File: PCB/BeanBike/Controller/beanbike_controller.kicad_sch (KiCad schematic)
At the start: 14 parts, among them SW1 SW_SPDT, U4 STM32G473RETx

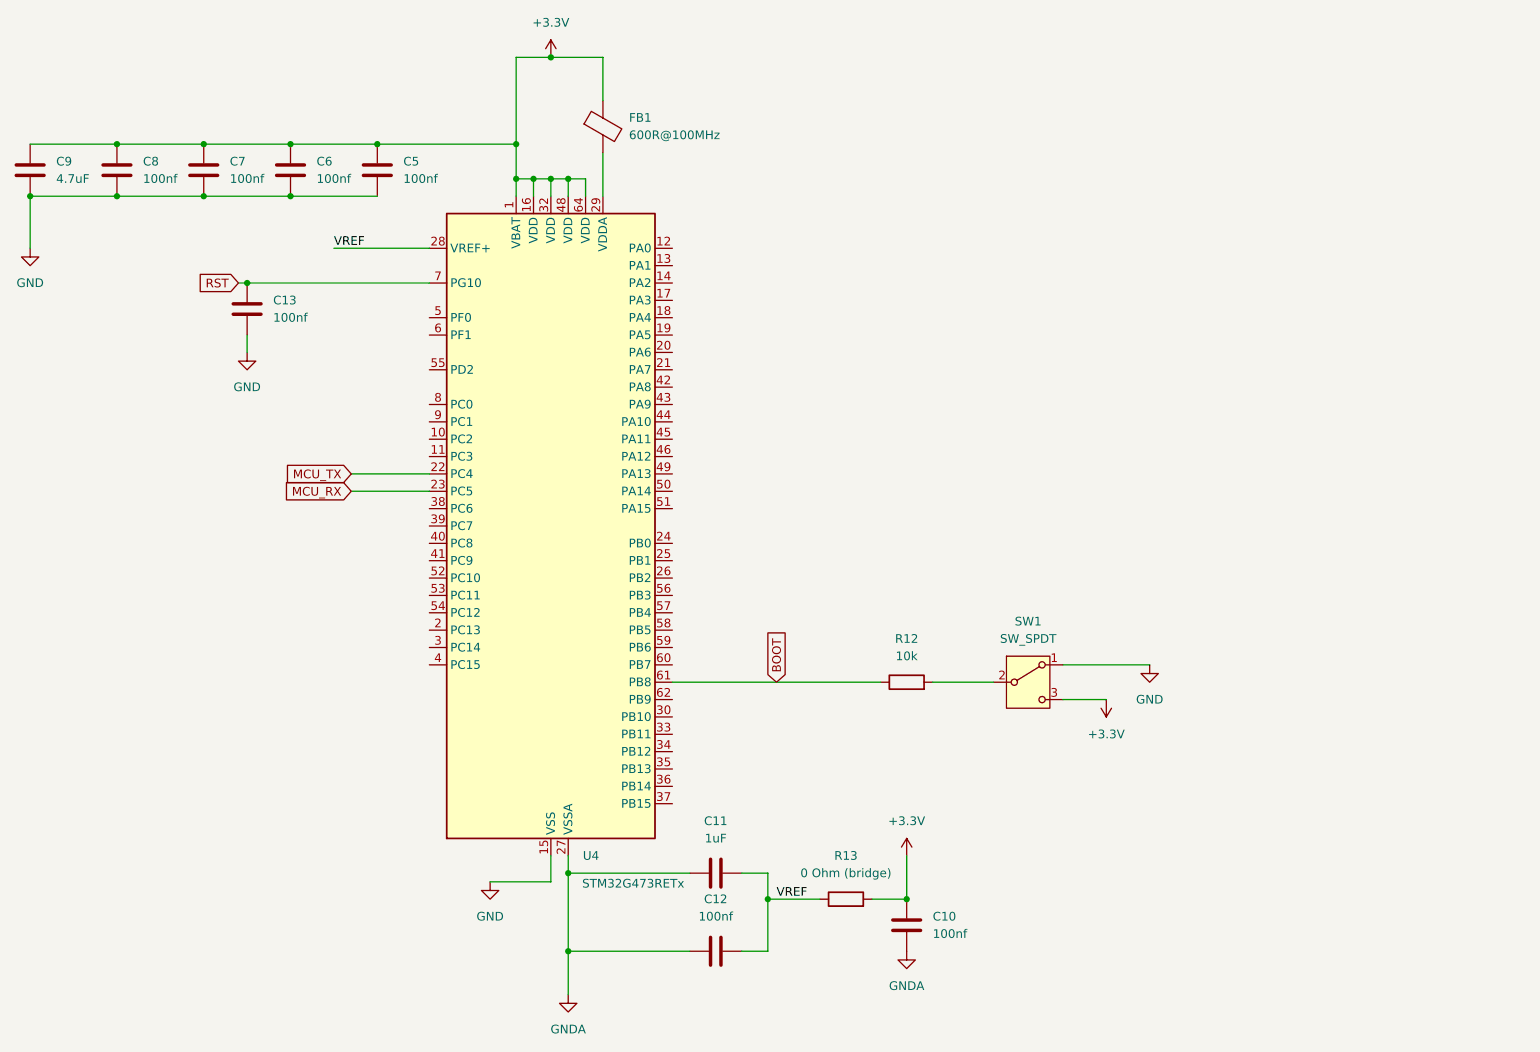
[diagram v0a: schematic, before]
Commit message: CAN
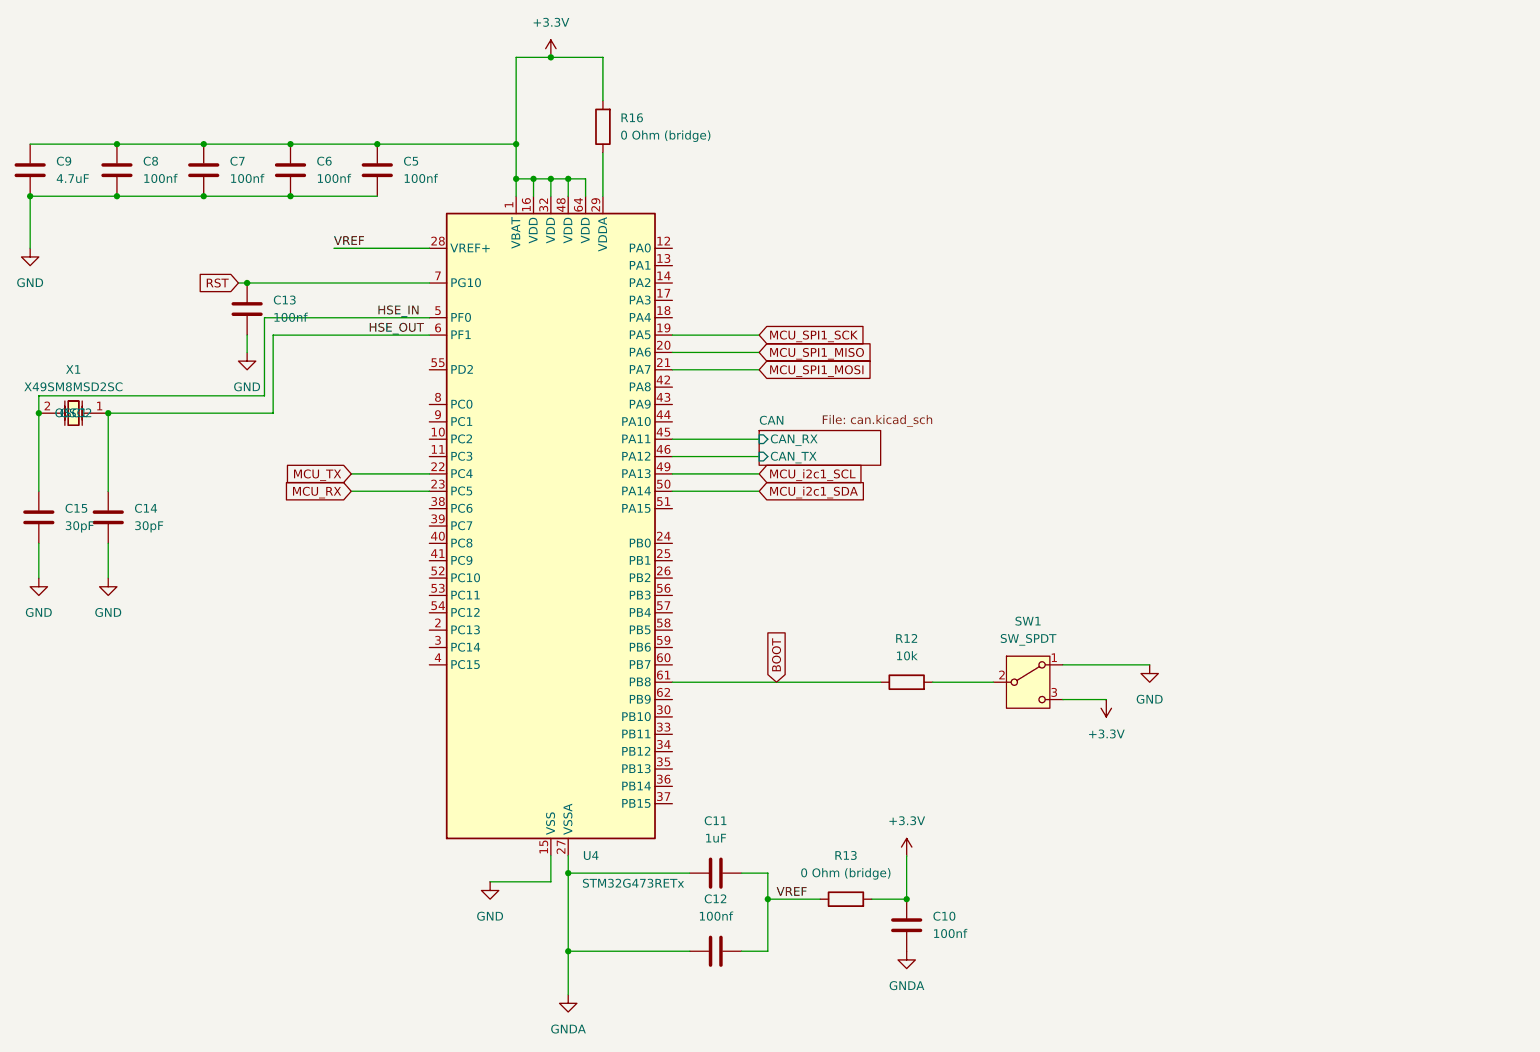
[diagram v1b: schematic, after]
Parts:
- removed FB1: 600R@100MHz, symbol Device:FerriteBead
- added C14, C15: 30pF, symbol Device:C
- added R16: 0 Ohm (bridge), symbol Device:R
- added X1: X49SM8MSD2SC, easyeda2kicad:CRYSTAL-SMD_L11.5-W4.8-LS12.7, symbol easyeda2kicad:X49SM8MSD2SC
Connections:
- net +3.3V: now also R16.2
- net GND: now also C14.2, C15.2
- net MCU_SPI1_SCK: now reaches U4.19 (PA5)
- net MCU_SPI1_MISO: now reaches U4.20 (PA6)
- net MCU_SPI1_MOSI: now reaches U4.21 (PA7)
- net at U4.29 (VDDA): now also R16.1
- net CAN/CAN_RX: now reaches U4.45 (PA11)
- net CAN/CAN_TX: now reaches U4.46 (PA12)
- net MCU_i2c1_SCL: now reaches U4.49 (PA13)
- net HSE_IN: now reaches U4.5 (PF0)
- net HSE_IN: now also C15.1, X1.2 (OSC2)
- net MCU_i2c1_SDA: now reaches U4.50 (PA14)
- net HSE_OUT: now reaches U4.6 (PF1)
- net HSE_OUT: now also C14.1, X1.1 (OSC1)
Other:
- added sheet CAN (can.kicad_sch)

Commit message: Schematic v3 Done
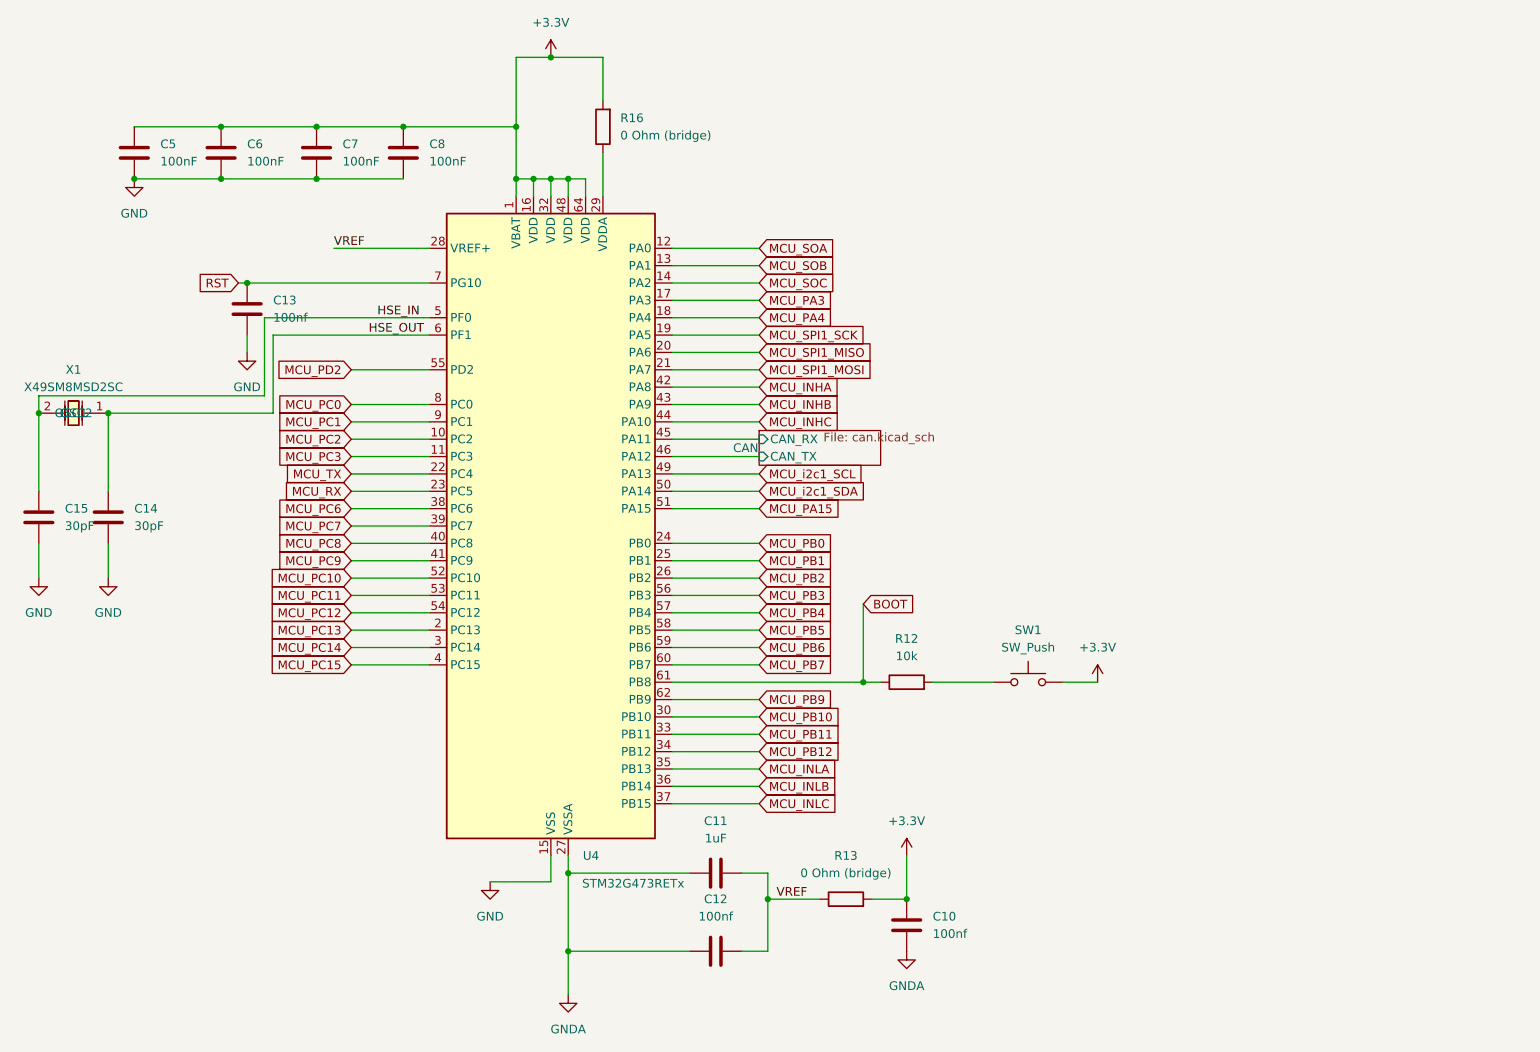
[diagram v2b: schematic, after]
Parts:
- removed C9: 4.7uF, symbol Device:C
- removed SW1: SW_SPDT, symbol Switch:SW_SPDT
- added SW1: SW_Push, symbol Switch:SW_Push
- C5, C6, C7, C8: value 100nf -> 100nF
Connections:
- net +3.3V: now also C5.2, C6.2, C7.2, C8.2, SW1.2; no longer C5.1, C6.1, C7.1, C8.1
- net GND: now also C5.1, C6.1, C7.1, C8.1; no longer C5.2, C6.2, C7.2, C8.2
- net at R12.2: now also SW1.1
- net MCU_PC2: now reaches U4.10 (PC2)
- net MCU_PC3: now reaches U4.11 (PC3)
- net MCU_SOA: now reaches U4.12 (PA0)
- net MCU_SOB: now reaches U4.13 (PA1)
- net MCU_SOC: now reaches U4.14 (PA2)
- net MCU_PA3: now reaches U4.17 (PA3)
- net MCU_PA4: now reaches U4.18 (PA4)
- net MCU_PC13: now reaches U4.2 (PC13)
- net MCU_PB0: now reaches U4.24 (PB0)
- net MCU_PB1: now reaches U4.25 (PB1)
- net MCU_PB2: now reaches U4.26 (PB2)
- net MCU_PC14: now reaches U4.3 (PC14)
- net MCU_PB10: now reaches U4.30 (PB10)
- net MCU_PB11: now reaches U4.33 (PB11)
- net MCU_PB12: now reaches U4.34 (PB12)
- net MCU_INLA: now reaches U4.35 (PB13)
- net MCU_INLB: now reaches U4.36 (PB14)
- net MCU_INLC: now reaches U4.37 (PB15)
- net MCU_PC6: now reaches U4.38 (PC6)
- net MCU_PC7: now reaches U4.39 (PC7)
- net MCU_PC15: now reaches U4.4 (PC15)
- net MCU_PC8: now reaches U4.40 (PC8)
- net MCU_PC9: now reaches U4.41 (PC9)
- net MCU_INHA: now reaches U4.42 (PA8)
- net MCU_INHB: now reaches U4.43 (PA9)
- net MCU_INHC: now reaches U4.44 (PA10)
- net MCU_PA15: now reaches U4.51 (PA15)
- net MCU_PC10: now reaches U4.52 (PC10)
- net MCU_PC11: now reaches U4.53 (PC11)
- net MCU_PC12: now reaches U4.54 (PC12)
- net MCU_PD2: now reaches U4.55 (PD2)
- net MCU_PB3: now reaches U4.56 (PB3)
- net MCU_PB4: now reaches U4.57 (PB4)
- net MCU_PB5: now reaches U4.58 (PB5)
- net MCU_PB6: now reaches U4.59 (PB6)
- net MCU_PB7: now reaches U4.60 (PB7)
- net MCU_PB9: now reaches U4.62 (PB9)
- net MCU_PC0: now reaches U4.8 (PC0)
- net MCU_PC1: now reaches U4.9 (PC1)

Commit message: Footprints
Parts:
- C10, C12, C13, C5, C6, C7, C8: footprint (none) -> Capacitor_SMD:C_0402_1005Metric; LCSC (none) -> C1525
- C11: footprint (none) -> Capacitor_SMD:C_0402_1005Metric; LCSC (none) -> C52923
- C14, C15: footprint (none) -> Capacitor_SMD:C_0402_1005Metric; LCSC (none) -> C1570
- R12: footprint (none) -> Resistor_SMD:R_0805_2012Metric; LCSC (none) -> C17414
- R13, R16: footprint (none) -> Resistor_SMD:R_0805_2012Metric; LCSC (none) -> C17477
- SW1: footprint (none) -> easyeda2kicad:SW-SMD_L3.9-W3.0-P4.45; LCSC (none) -> C720477
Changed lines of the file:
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@@
 			)
 		)
-		(property "Footprint" ""
+		(property "Footprint" "easyeda2kicad:SW-SMD_L3.9-W3.0-P4.45"
 			(at 207.01 118.11 0)
 			(effects
@@
 			)
 		)
+		(property "LCSC" "C720477"
+			(at 207.01 123.19 0)
+			(effects
+				(font
+					(size 1.27 1.27)
+				)
+				(hide yes)
+			)
+		)
 		(pin "1"
 		)
@@
 			)
 		)
-		(property "Footprint" ""
+		(property "Footprint" "Capacitor_SMD:C_0402_1005Metric"
 			(at 75.2348 41.91 0)
 			(effects
@@
 			)
 		)
+		(property "LCSC" "C1525"
+			(at 76.2 45.72 0)
+			(effects
+				(font
+					(size 1.27 1.27)
+				)
+				(hide yes)
+			)
+		)
 		(pin "1"
 		)
@@
 			)
 		)
-		(property "Footprint" ""
+		(property "Footprint" "Capacitor_SMD:C_0402_1005Metric"
 			(at 114.6048 41.91 0)
 			(effects
@@
 			)
 		)
+		(property "LCSC" "C1525"
+			(at 115.57 45.72 0)
+			(effects
+				(font
+					(size 1.27 1.27)
+				)
+				(hide yes)
+			)
+		)
 		(pin "1"
 		)
@@
 			)
 		)
-		(property "Footprint" ""
+		(property "Footprint" "Resistor_SMD:R_0805_2012Metric"
 			(at 146.558 41.91 90)
 			(effects
@@
 			)
 		)
+		(property "LCSC" "C17477"
+			(at 144.78 41.91 0)
+			(effects
+				(font
+					(size 1.27 1.27)
+				)
+				(hide yes)
+			)
+		)
 		(pin "1"
 		)
@@
 			)
 		)
-		(property "Footprint" ""
+		(property "Footprint" "Capacitor_SMD:C_0402_1005Metric"
 			(at 165.1 150.1648 0)
 			(effects
@@
 			)
 		)
+		(property "LCSC" "C52923"
+			(at 161.29 151.13 90)
+			(effects
+				(font
+					(size 1.27 1.27)
+				)
+				(hide yes)
+			)
+		)
 		(pin "2"
 		)
@@
 			)
 		)
-		(property "Footprint" ""
+		(property "Footprint" "Capacitor_SMD:C_0402_1005Metric"
 			(at 63.1952 102.87 0)
 			(effects
@@
 			)
 		)
+		(property "LCSC" "C1570"
+			(at 62.23 99.06 0)
+			(effects
+				(font
+					(size 1.27 1.27)
+				)
+				(hide yes)
+			)
+		)
 		(pin "1"
 		)
@@
 			)
 		)
-		(property "Footprint" ""
+		(property "Footprint" "Capacitor_SMD:C_0402_1005Metric"
 			(at 87.9348 41.91 0)
 			(effects
@@
 			)
 		)
+		(property "LCSC" "C1525"
+			(at 88.9 45.72 0)
+			(effects
+				(font
+					(size 1.27 1.27)
+				)
+				(hide yes)
+			)
+		)
 		(pin "1"
 		)
@@
 			)
 		)
-		(property "Footprint" ""
+		(property "Footprint" "Resistor_SMD:R_0805_2012Metric"
 			(at 189.23 124.968 90)
 			(effects
@@
 			)
 		)
+		(property "LCSC" "C17414"
+			(at 189.23 123.19 90)
+			(effects
+				(font
+					(size 1.27 1.27)
+				)
+				(hide yes)
+			)
+		)
 		(pin "2"
 		)
@@
 			)
 		)
-		(property "Footprint" ""
+		(property "Footprint" "Capacitor_SMD:C_0402_1005Metric"
 			(at 93.6752 72.39 0)
 			(effects
@@
 			)
 		)
+		(property "LCSC" "C1525"
+			(at 92.71 68.58 0)
+			(effects
+				(font
+					(size 1.27 1.27)
+				)
+				(hide yes)
+			)
+		)
 		(pin "1"
 		)
@@
 			)
 		)
-		(property "Footprint" ""
+		(property "Footprint" "Capacitor_SMD:C_0402_1005Metric"
 			(at 101.9048 41.91 0)
 			(effects
@@
 			)
 		)
+		(property "LCSC" "C1525"
+			(at 102.87 45.72 0)
+			(effects
+				(font
+					(size 1.27 1.27)
+				)
+				(hide yes)
+			)
+		)
 		(pin "1"
 		)
@@
 			)
 		)
-		(property "Footprint" ""
+		(property "Footprint" "Resistor_SMD:R_0805_2012Metric"
 			(at 180.34 156.718 90)
 			(effects
@@
 			)
 		)
+		(property "LCSC" "C17477"
+			(at 180.34 154.94 90)
+			(effects
+				(font
+					(size 1.27 1.27)
+				)
+				(hide yes)
+			)
+		)
 		(pin "1"
 		)
@@
 			)
 		)
-		(property "Footprint" ""
+		(property "Footprint" "Capacitor_SMD:C_0402_1005Metric"
 			(at 73.3552 102.87 0)
 			(effects
@@
 			)
 		)
+		(property "LCSC" "C1570"
+			(at 72.39 99.06 0)
+			(effects
+				(font
+					(size 1.27 1.27)
+				)
+				(hide yes)
+			)
+		)
 		(pin "1"
 		)
@@
 			)
 		)
-		(property "Footprint" ""
+		(property "Footprint" "Capacitor_SMD:C_0402_1005Metric"
 			(at 165.1 161.5948 0)
 			(effects
@@
 			)
 		)
+		(property "LCSC" "C1525"
+			(at 161.29 162.56 90)
+			(effects
+				(font
+					(size 1.27 1.27)
+				)
+				(hide yes)
+			)
+		)
 		(pin "2"
 		)
@@
 			)
 		)
-		(property "Footprint" ""
+		(property "Footprint" "Capacitor_SMD:C_0402_1005Metric"
 			(at 190.1952 162.56 0)
 			(effects
@@
 			(at 189.23 158.75 0)
 			(effects
+				(font
+					(size 1.27 1.27)
+				)
+				(hide yes)
+			)
+		)
+		(property "LCSC" "C1525"
+			(at 189.23 158.75 0)
+			(effects
